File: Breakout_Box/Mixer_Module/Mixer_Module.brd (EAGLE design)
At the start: 47 x 66 mm, 130 parts, among them T1 2SC3324, T10 2SC3324, T11 2SC3324, T12 2SC3324, T13 2N4401, T2 2SC3324, T3 2SC3324, T4 2SC3324, T5 2SC3324, T6 2SC3324, T7 2SC3324, T8 2SC3324, T9 2SC3324, U1 OPA2209, U2 MCP10804-T

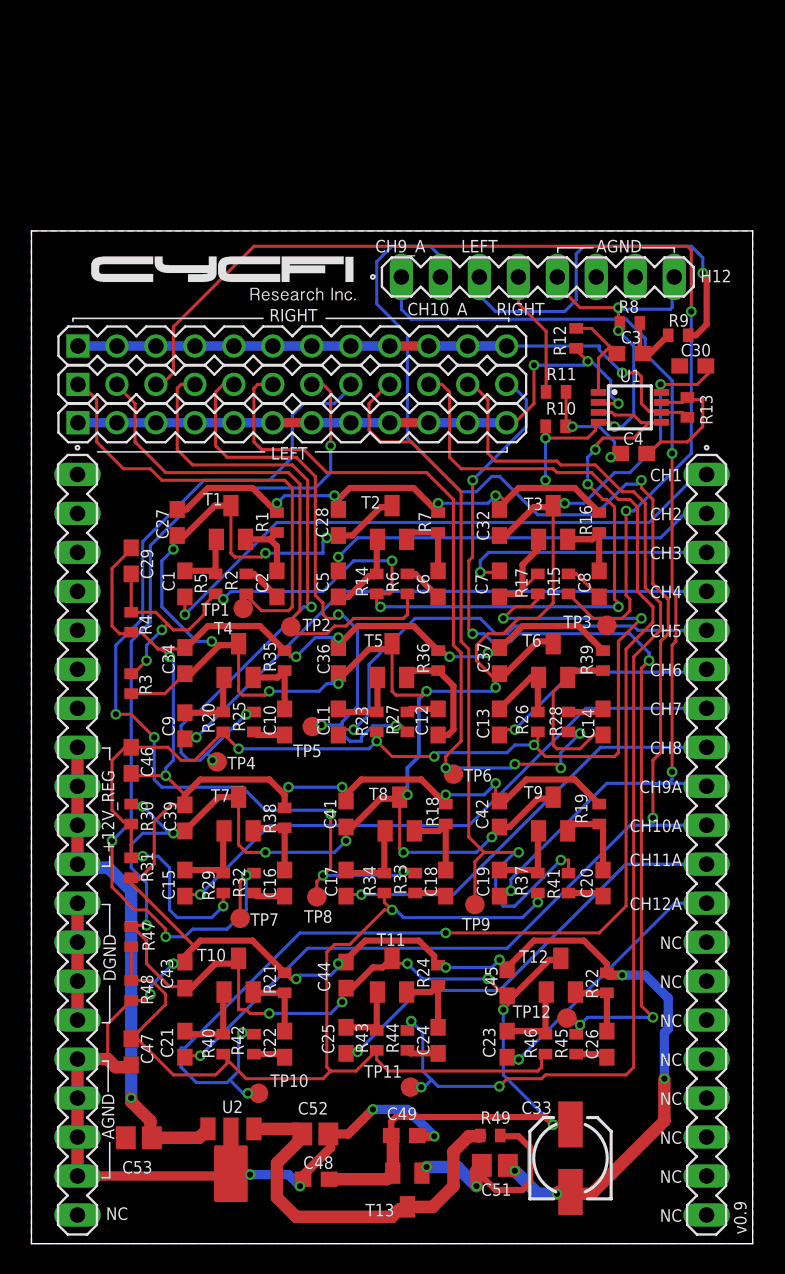
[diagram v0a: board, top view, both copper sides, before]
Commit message: Licenses
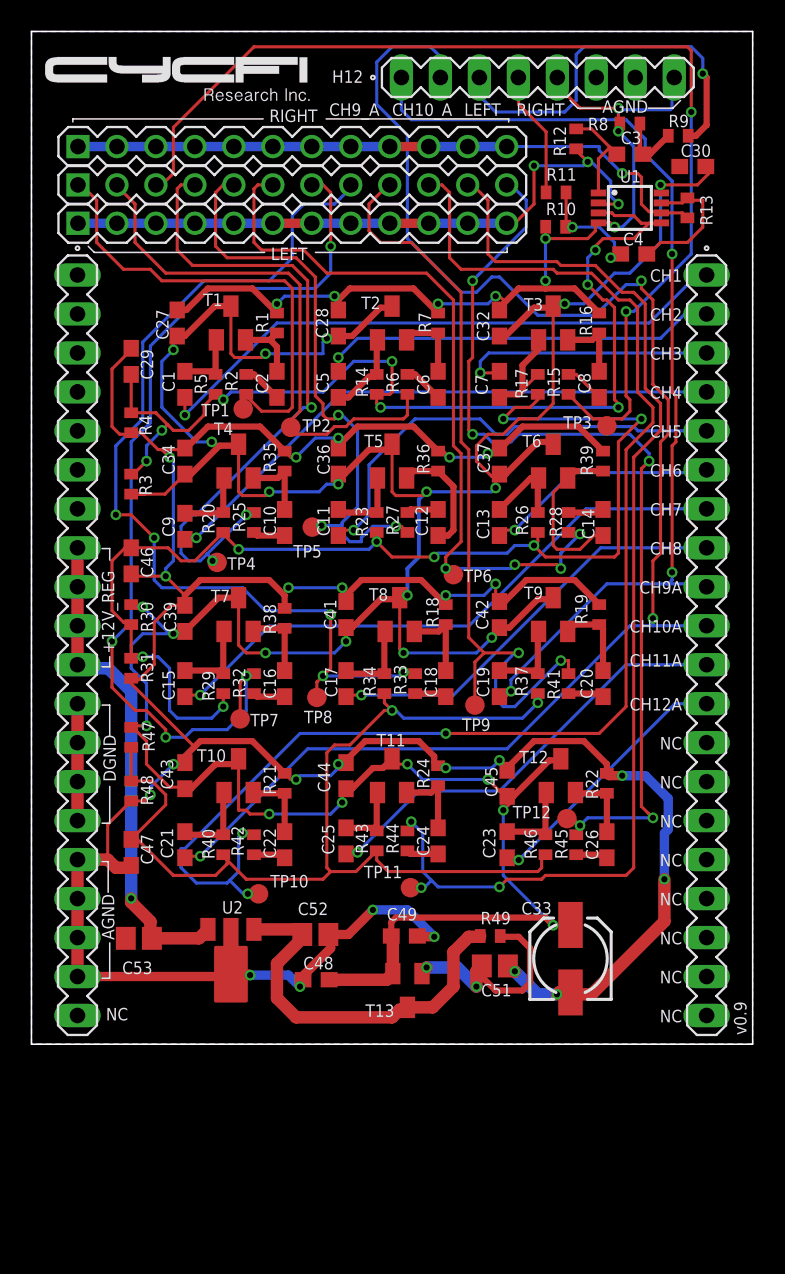
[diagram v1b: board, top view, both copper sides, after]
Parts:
- moved R11 13.0 mm to (34.2, 68.5)
- moved TP7 13.0 mm to (13.6, 34.2)
- moved C51 13.0 mm to (30.2, 18.1)
- moved C1 13.0 mm to (10.0, 56.0)
- moved C10 13.0 mm to (16.5, 47.0)
- moved C11 13.0 mm to (20.0, 47.0)
- moved C12 13.0 mm to (26.5, 47.0)
- moved C13 13.0 mm to (30.5, 47.0)
- moved C14 13.0 mm to (37.2, 47.0)
- moved C15 13.0 mm to (10.0, 36.5)
- moved C16 13.0 mm to (16.5, 36.5)
- moved C17 13.0 mm to (20.5, 36.5)
- moved C18 13.0 mm to (27.0, 36.5)
- moved C19 13.0 mm to (30.5, 36.5)
- moved C2 13.0 mm to (16.0, 56.0)
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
